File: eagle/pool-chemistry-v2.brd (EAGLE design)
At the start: 38.7 x 29.8 mm, 17 parts, among them U1 ESP-WROOM-32

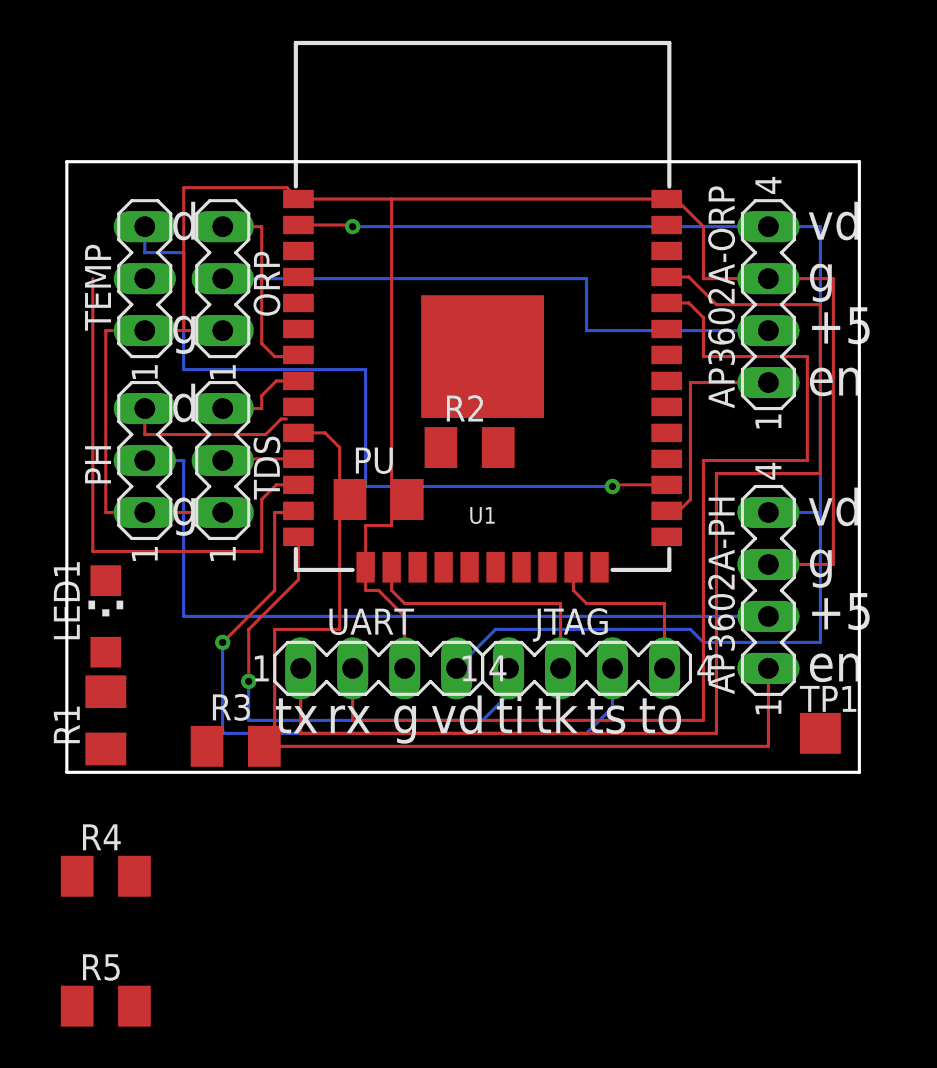
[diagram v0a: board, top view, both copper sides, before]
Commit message: discrete components placed and routed
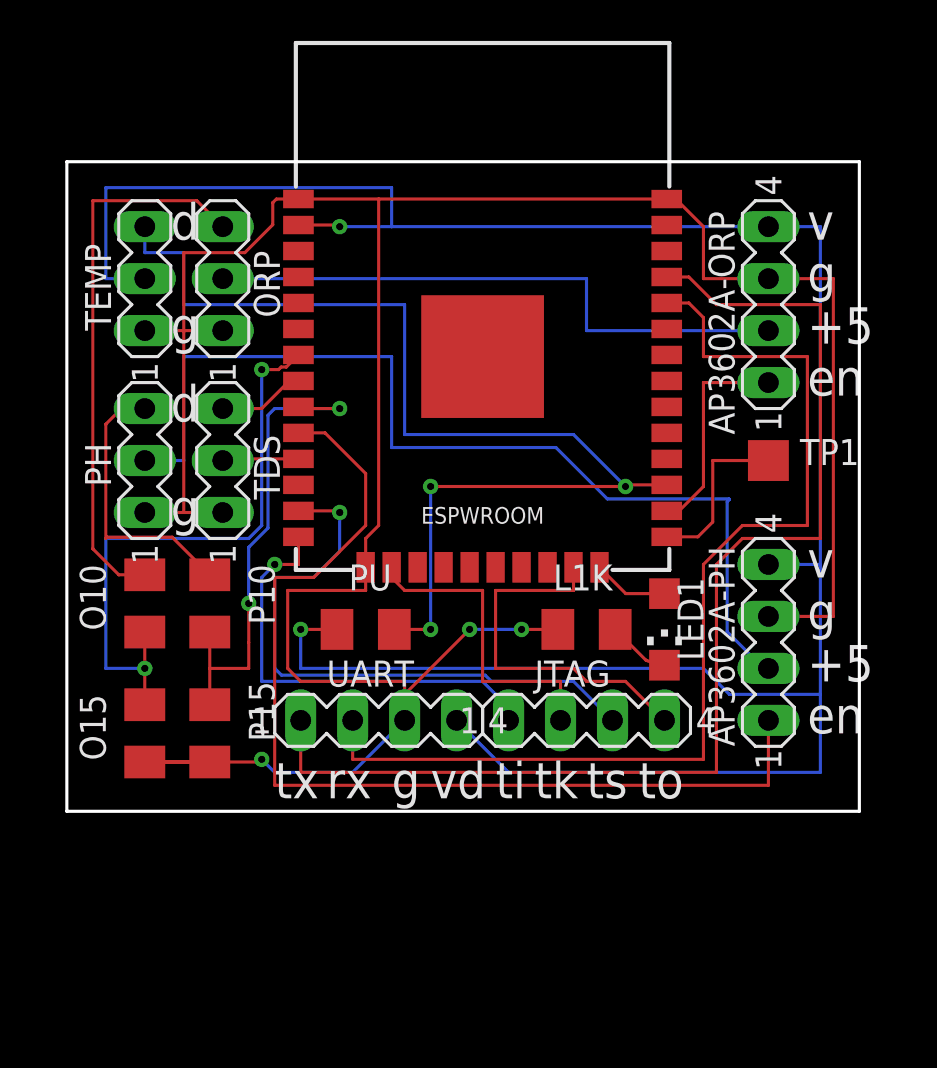
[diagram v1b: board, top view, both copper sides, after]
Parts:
- removed R1: 1k, rcl:M1206
- removed R2, R5: 10k, rcl:M1206
- removed R3, R4: 15k, rcl:M1206
- added L1K: 1k, rcl:M1206
- added O10, P10: 10k, rcl:M1206
- added O15, P15: 15k, rcl:M1206
- moved LED1 27.3 mm to (34.3, 8.26), turned to 180 degrees
- moved TP1 13.6 mm to (39.4, 16.5)
- moved PU 6.38 mm to (19.7, 8.26), turned to 180 degrees
- moved AP3602A-PH 2.54 mm to (39.4, 7.62)
- moved JTAG 2.54 mm to (30.5, 3.81)
- moved UART 2.54 mm to (20.3, 3.81)
- renumbered U1 to ESPWROOM
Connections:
- removed net TEMPEN: ESPWROOM.12, PU.1
- net GND: now also L1K.2, O15.2, P15.2; no longer R1.2, R3.2, R4.2
- net N$1: now also L1K.1; no longer R1.1
- net N$2: now also O10.2, O15.1; no longer R2.2, R3.1
- net N$4: now also P10.2, P15.1; no longer R4.1, R5.2
- net ORPSIG: now also O10.1; no longer R2.1
- net PHSIG: now also P10.1; no longer R5.1
- net TEMPSIG: now also PU.1; no longer PU.2
- net VDD: now also PU.2
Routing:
- net VDD: track 67.2 -> 125.4 mm, vias 1 -> 2
- net GND: track 104.9 -> 137.5 mm, vias 0 -> 3
- net N$2: track 0.00 -> 29.4 mm, vias 0 -> 2
- net TEMPEN: track 26.2 -> 0.00 mm
- net N$4: track 0.00 -> 23.9 mm, vias 0 -> 2
- net ORPSIG: track 9.60 -> 27.0 mm
- net TEMPSIG: track 38.2 -> 55.0 mm, vias 1 -> 3
- net PH+5: track 38.1 -> 48.4 mm
- net TDO: track 9.01 -> 18.1 mm
- net TOUCH: track 0.00 -> 8.28 mm
- net PHSIG: track 8.50 -> 13.7 mm
- net TMS: track 34.5 -> 29.7 mm
- net LED: track 0.00 -> 3.71 mm
- net N$1: track 0.00 -> 3.08 mm
- net TDI: track 24.5 -> 21.7 mm
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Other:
- board size 38.7 x 29.8 mm -> 38.7 x 31.8 mm
- board text added: "v"

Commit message: added missing labels to voltage divided signals
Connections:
- removed net N$2: ESPWROOM.7, O10.2, O15.1
- removed net N$4: ESPWROOM.9, P10.2, P15.1
- net ORPSIG: now also ESPWROOM.7, O10.2, O15.1
- net PHSIG: now also ESPWROOM.9, P10.2, P15.1
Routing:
- net N$2: track 29.4 -> 0.00 mm, vias 2 -> 0
- net ORPSIG: track 27.0 -> 56.4 mm, vias 0 -> 2
- net PHSIG: track 13.7 -> 37.6 mm, vias 0 -> 2
- net N$4: track 23.9 -> 0.00 mm, vias 2 -> 0
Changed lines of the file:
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@@
 <wire x1="12.7" y1="27.94" x2="11.43" y2="29.21" width="0.1524" layer="1"/>
 <wire x1="11.43" y1="29.21" x2="6.35" y2="29.21" width="0.1524" layer="1"/>
+<contactref element="ESPWROOM" pad="7"/>
+<contactref element="O10" pad="2"/>
+<contactref element="O15" pad="1"/>
+<wire x1="8.89" y1="8.125" x2="8.89" y2="6.35" width="0.1524" layer="1"/>
+<wire x1="8.89" y1="6.35" x2="8.89" y2="4.575" width="0.1524" layer="1"/>
+<wire x1="16.4" y1="21.67" x2="15.8086" y2="21.0786" width="0.1524" layer="1"/>
+<wire x1="15.8086" y1="21.0786" x2="15.5553125" y2="21.0786" width="0.1524" layer="1"/>
+<wire x1="15.5553125" y1="21.0786" x2="15.4317125" y2="20.955" width="0.1524" layer="1"/>
+<wire x1="15.4317125" y1="20.955" x2="14.605" y2="20.955" width="0.1524" layer="1"/>
+<via x="14.605" y="20.955" extent="1-16" drill="0.35"/>
+<wire x1="14.605" y1="20.955" x2="14.605" y2="13.335" width="0.1524" layer="16"/>
+<wire x1="14.605" y1="13.335" x2="13.97" y2="12.7" width="0.1524" layer="16"/>
+<wire x1="13.97" y1="12.7" x2="6.985" y2="12.7" width="0.1524" layer="16"/>
+<via x="8.89" y="6.35" extent="1-16" drill="0.35"/>
+<wire x1="6.985" y1="6.35" x2="8.89" y2="6.35" width="0.1524" layer="16"/>
+<wire x1="6.985" y1="12.7" x2="6.985" y2="6.35" width="0.1524" layer="16"/>
+<wire x1="8.89" y1="8.125" x2="8.89" y2="10.925" width="0" layer="19" extent="1-1"/>
 </signal>
 <signal name="TDSSIG">
@@
 <wire x1="6.985" y1="12.7" x2="6.985" y2="18.285" width="0.1524" layer="1"/>
 <wire x1="6.985" y1="18.285" x2="7.75" y2="19.05" width="0.1524" layer="1"/>
+<contactref element="ESPWROOM" pad="9"/>
+<contactref element="P10" pad="2"/>
+<contactref element="P15" pad="1"/>
+<wire x1="12.065" y1="8.125" x2="12.065" y2="6.35" width="0.1524" layer="1"/>
+<wire x1="12.065" y1="6.35" x2="12.065" y2="4.575" width="0.1524" layer="1"/>
+<wire x1="13.97" y1="7.62" x2="13.97" y2="9.525" width="0.1524" layer="1"/>
+<via x="13.97" y="9.525" extent="1-16" drill="0.35"/>
+<wire x1="13.97" y1="9.525" x2="13.97" y2="12.26894375" width="0.1524" layer="16"/>
+<wire x1="13.97" y1="12.26894375" x2="14.9098" y2="13.20874375" width="0.1524" layer="16"/>
+<wire x1="14.9098" y1="18.7198" x2="15.24" y2="19.05" width="0.1524" layer="16"/>
+<wire x1="14.9098" y1="13.20874375" x2="14.9098" y2="18.7198" width="0.1524" layer="16"/>
+<wire x1="15.24" y1="19.05" x2="18.415" y2="19.05" width="0.1524" layer="16"/>
+<via x="18.415" y="19.05" extent="1-16" drill="0.35"/>
+<wire x1="18.415" y1="19.05" x2="16.48" y2="19.05" width="0.1524" layer="1"/>
+<wire x1="16.48" y1="19.05" x2="16.4" y2="19.13" width="0.1524" layer="1"/>
+<wire x1="12.065" y1="6.35" x2="13.97" y2="6.35" width="0.1524" layer="1"/>
+<wire x1="13.97" y1="6.35" x2="13.97" y2="7.62" width="0.1524" layer="1"/>
+<wire x1="13.97" y1="9.525" x2="12.065" y2="10.925" width="0" layer="19" extent="1-1"/>
 </signal>
 <signal name="TX">
@@
 <wire x1="33.994259375" y1="6.505" x2="33.381475" y2="6.753525" width="0.1524" layer="1"/>
 </signal>
-<signal name="N$2">
-<contactref element="ESPWROOM" pad="7"/>
-<contactref element="O10" pad="2"/>
-<contactref element="O15" pad="1"/>
-<wire x1="8.89" y1="8.125" x2="8.89" y2="6.35" width="0.1524" layer="1"/>
-<wire x1="8.89" y1="6.35" x2="8.89" y2="4.575" width="0.1524" layer="1"/>
-<wire x1="16.4" y1="21.67" x2="15.8086" y2="21.0786" width="0.1524" layer="1"/>
-<wire x1="15.8086" y1="21.0786" x2="15.5553125" y2="21.0786" width="0.1524" layer="1"/>
-<wire x1="15.5553125" y1="21.0786" x2="15.4317125" y2="20.955" width="0.1524" layer="1"/>
-<wire x1="15.4317125" y1="20.955" x2="14.605" y2="20.955" width="0.1524" layer="1"/>
-<via x="14.605" y="20.955" extent="1-16" drill="0.35"/>
-<wire x1="14.605" y1="20.955" x2="14.605" y2="13.335" width="0.1524" layer="16"/>
-<wire x1="14.605" y1="13.335" x2="13.97" y2="12.7" width="0.1524" layer="16"/>
-<wire x1="13.97" y1="12.7" x2="6.985" y2="12.7" width="0.1524" layer="16"/>
-<via x="8.89" y="6.35" extent="1-16" drill="0.35"/>
-<wire x1="6.985" y1="6.35" x2="8.89" y2="6.35" width="0.1524" layer="16"/>
-<wire x1="6.985" y1="12.7" x2="6.985" y2="6.35" width="0.1524" layer="16"/>
-</signal>
-<signal name="N$4">
-<contactref element="ESPWROOM" pad="9"/>
-<contactref element="P10" pad="2"/>
-<contactref element="P15" pad="1"/>
-<wire x1="12.065" y1="8.125" x2="12.065" y2="6.35" width="0.1524" layer="1"/>
-<wire x1="12.065" y1="6.35" x2="12.065" y2="4.575" width="0.1524" layer="1"/>
-<wire x1="13.97" y1="7.62" x2="13.97" y2="9.525" width="0.1524" layer="1"/>
-<via x="13.97" y="9.525" extent="1-16" drill="0.35"/>
-<wire x1="13.97" y1="9.525" x2="13.97" y2="12.26894375" width="0.1524" layer="16"/>
-<wire x1="13.97" y1="12.26894375" x2="14.9098" y2="13.20874375" width="0.1524" layer="16"/>
-<wire x1="14.9098" y1="18.7198" x2="15.24" y2="19.05" width="0.1524" layer="16"/>
-<wire x1="14.9098" y1="13.20874375" x2="14.9098" y2="18.7198" width="0.1524" layer="16"/>
-<wire x1="15.24" y1="19.05" x2="18.415" y2="19.05" width="0.1524" layer="16"/>
-<via x="18.415" y="19.05" extent="1-16" drill="0.35"/>
-<wire x1="18.415" y1="19.05" x2="16.48" y2="19.05" width="0.1524" layer="1"/>
-<wire x1="16.48" y1="19.05" x2="16.4" y2="19.13" width="0.1524" layer="1"/>
-<wire x1="12.065" y1="6.35" x2="13.97" y2="6.35" width="0.1524" layer="1"/>
-<wire x1="13.97" y1="6.35" x2="13.97" y2="7.62" width="0.1524" layer="1"/>
-</signal>
 </signals>
